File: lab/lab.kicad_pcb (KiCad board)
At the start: 2 copper layers, 45.7 x 31.8 mm, 42 parts, among them J1 FACE, J3 C?, Q1 Q_NPN_EBC, Q2 Q_NPN_EBC, Q3 Q_NPN_EBC, U1 LM324, U2 L78L33_TO92

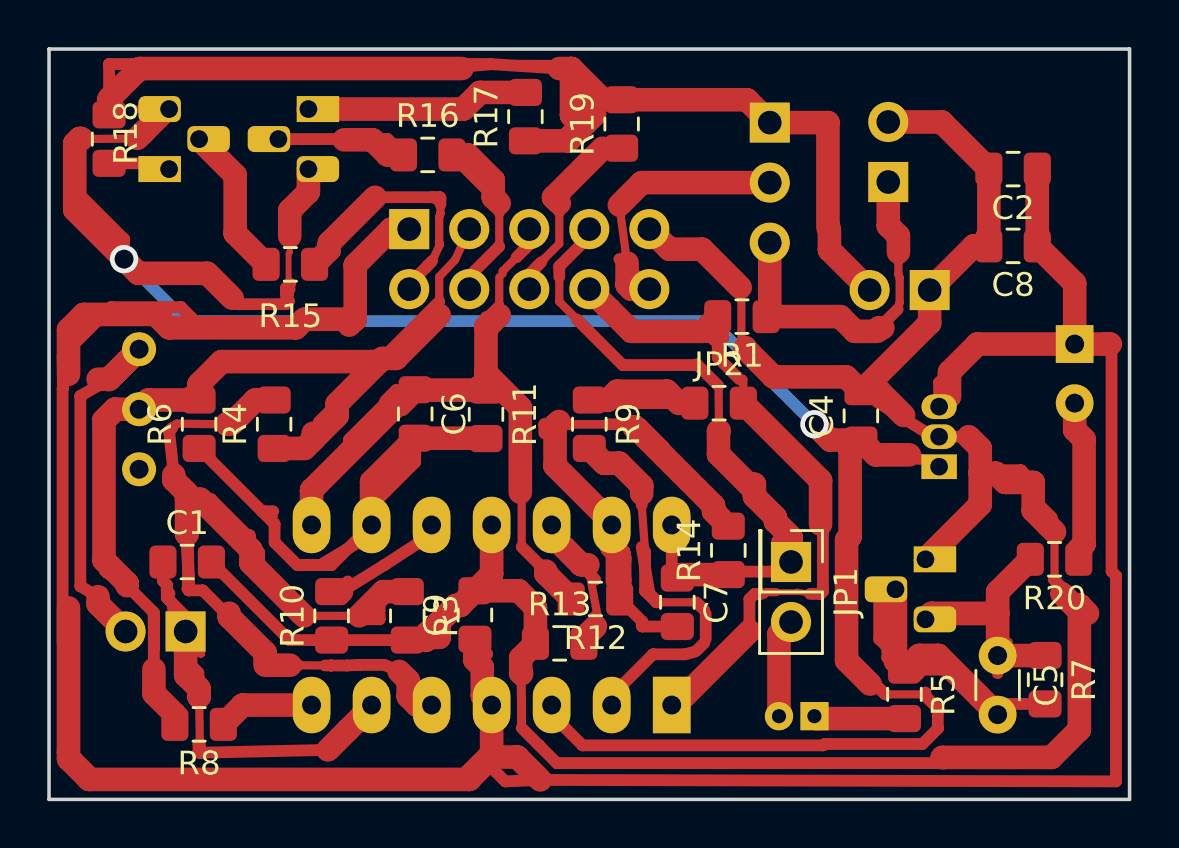
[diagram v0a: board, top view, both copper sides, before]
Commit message: as of today
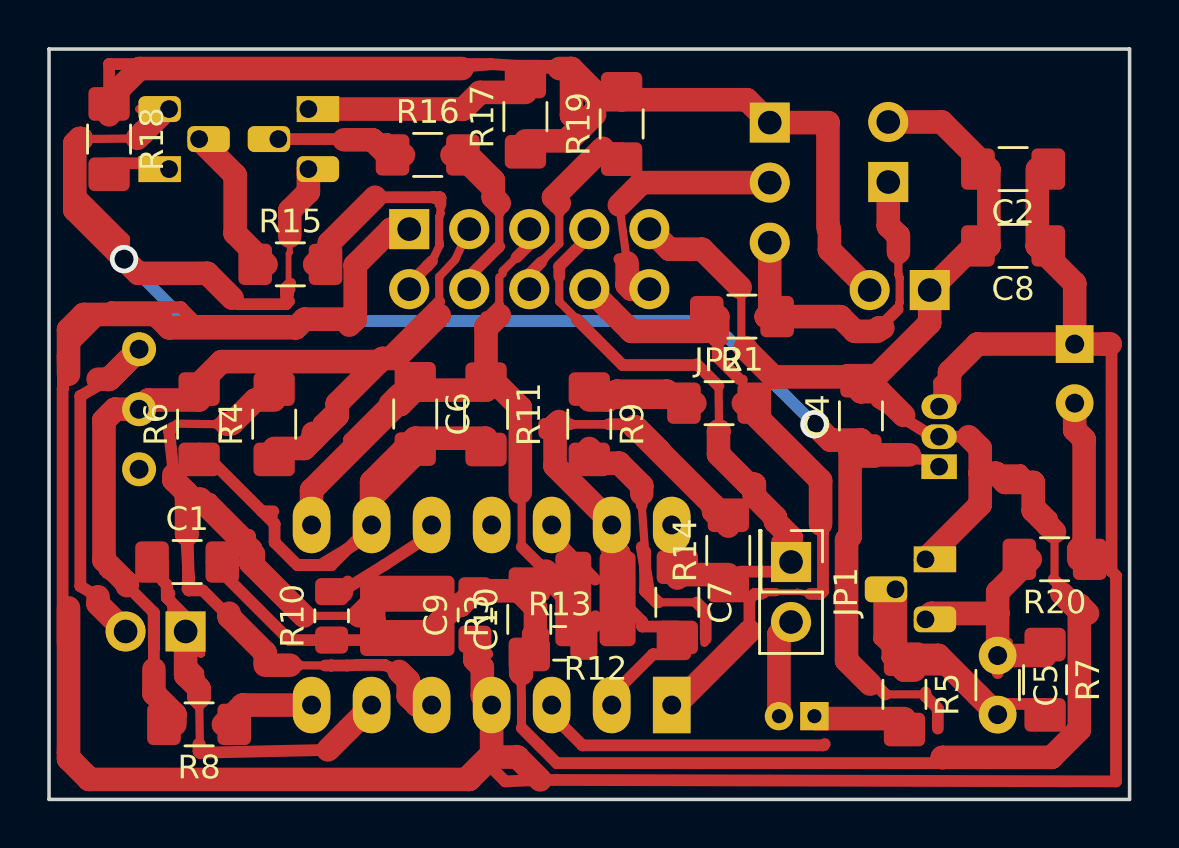
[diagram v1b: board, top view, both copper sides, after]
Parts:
- added C10: 100n, Capacitor_SMD:C_1206_3216Metric_Pad1.42x1.75mm_HandSolder, F.Cu at (39.4, 41.9)
- C1, C2, C4, C6, C7, C8: footprint Capacitor_SMD:C_0805_2012Metric_Pad1.15x1.40mm_HandSolder -> Capacitor_SMD:C_1206_3216Metric_Pad1.42x1.75mm_HandSolder
- JP2, R1, R11, R14, R15, R16, R17, R18, R19, R20, R4, R5, R6, R7, R8, R9: footprint Resistor_SMD:R_0805_2012Metric_Pad1.15x1.40mm_HandSolder -> Resistor_SMD:R_1206_3216Metric_Pad1.42x1.75mm_HandSolder
- R12, R3: footprint Resistor_SMD:R_0805_2012Metric_Pad1.15x1.40mm_HandSolder -> Resistor_SMD:R_0815_2038Metric_Pad1.53x4.00mm_HandSolder
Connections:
- U1 pad 11: GNDD -> -5V
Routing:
- net Net-(R13-Pad2): track 11.5 -> 4.53 mm
- net 3V3: track 119.1 -> 114.1 mm
- net GNDD: track 127.9 -> 124.8 mm
- net CMEAS: track 103.6 -> 101.9 mm
- net Net-(R9-Pad2): track 19.6 -> 18.6 mm
